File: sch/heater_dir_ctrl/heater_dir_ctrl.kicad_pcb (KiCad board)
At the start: 2 copper layers, 88 parts, among them J1 JMP1, J10 heater, J11 heater, J2 JMP1, J3 UV, J4 SWD, J5 motor, J6 motor, J7 ., J8 ac_in, J9 ac_in, Q1 AO3400, Q2 DTD114E, Q3 Q_Photo_NPN_CE, Q4 2N60, Q5 2N60, Q6 2N60, Q7 2N60, Q8 DTD114E, Q9 DTD114E, SW1 SW_Push, SW2 SW_Push, U1 STM32F031F4P6, U2 LNK306D, U3 AP1117-33, U4 TM1637, U5 IRS2103, U6 LTV-817, U8 IRS2103

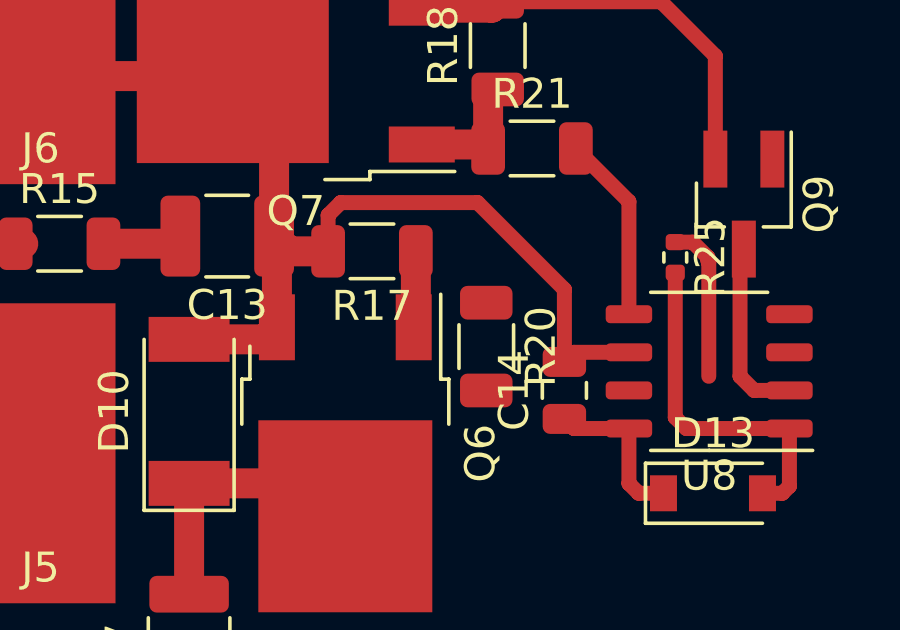
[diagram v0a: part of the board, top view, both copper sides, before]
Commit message: commas
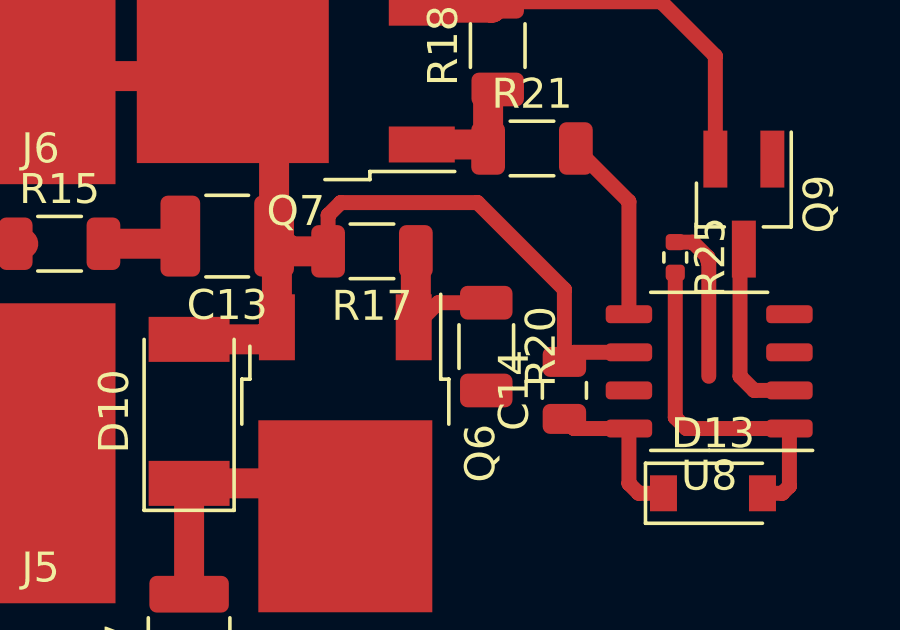
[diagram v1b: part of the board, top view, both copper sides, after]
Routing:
- net Net-(Q6-Pad1): track 2.56 -> 5.32 mm

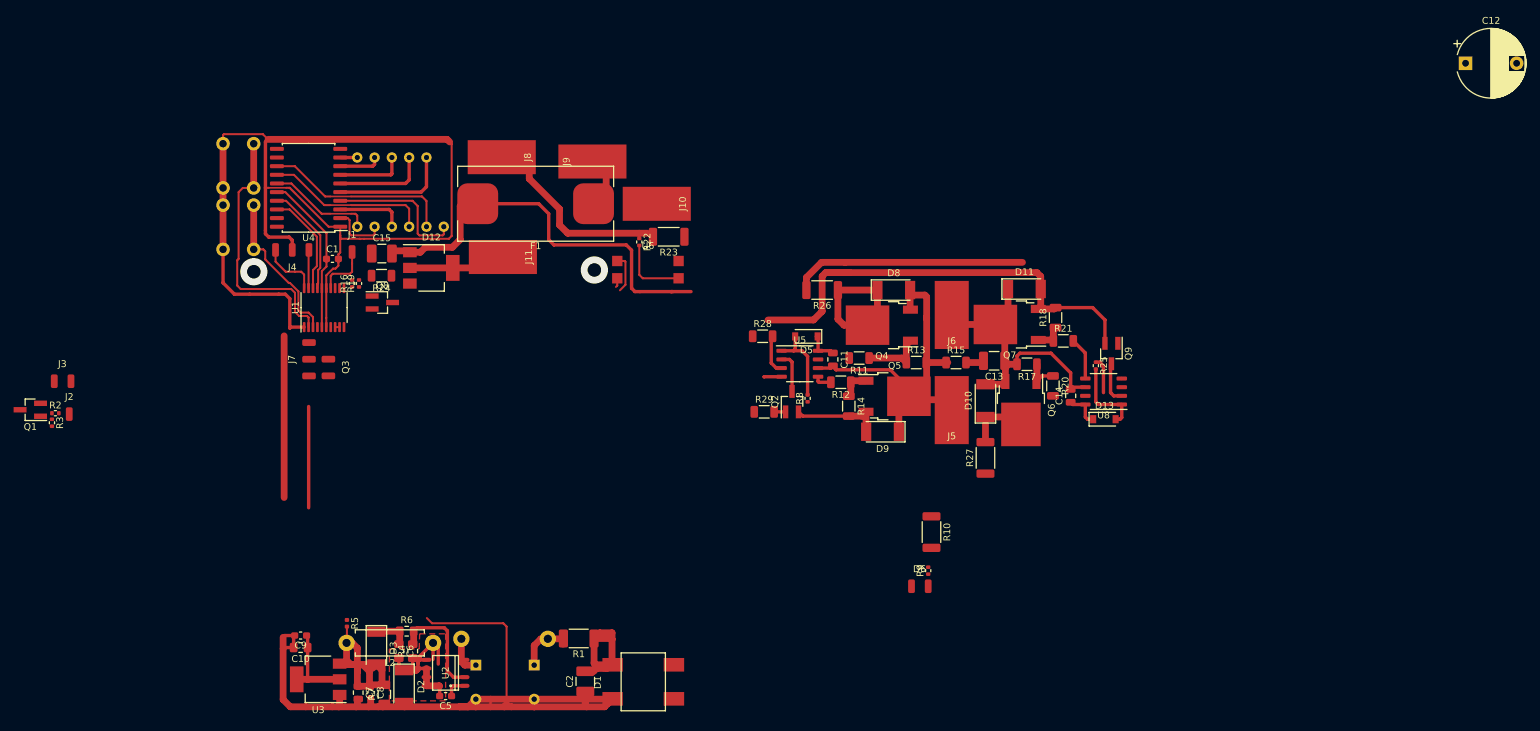
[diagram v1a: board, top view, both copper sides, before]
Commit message: board ok
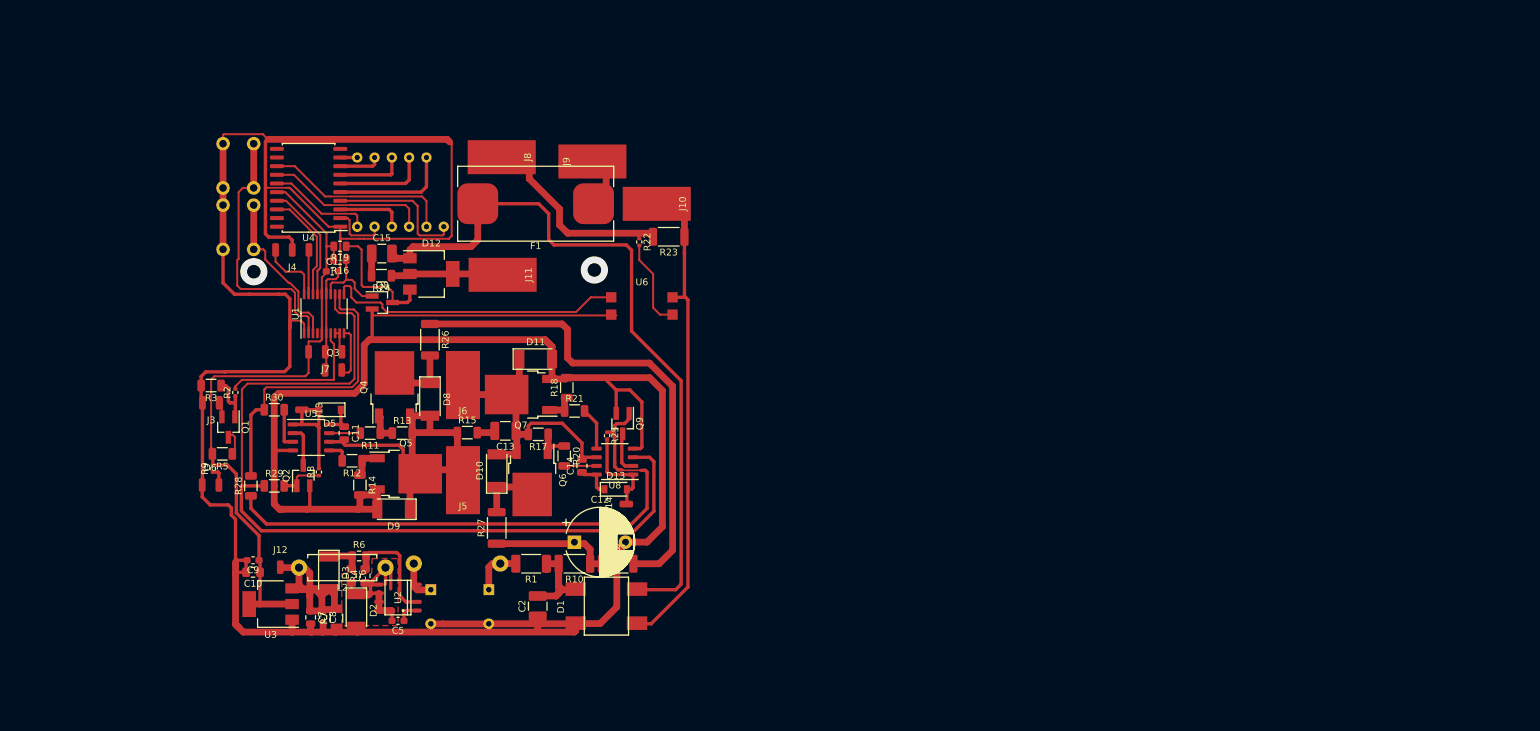
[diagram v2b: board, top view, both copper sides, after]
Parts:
- removed J1, J2: JMP1, Connector_Wire:SolderWirePad_1x01_SMD_1x2mm
- added J12: 10V, Connector_Wire:SolderWirePad_1x01_SMD_1x2mm, F.Cu at (111.9, 125.2)
- added J13: 10V, Connector_Wire:SolderWirePad_1x01_SMD_1x2mm, F.Cu at (115.1, 102.1)
- added J14: 10V, Connector_Wire:SolderWirePad_1x01_SMD_1x2mm, F.Cu at (162.7, 116.0)
- added R30: 220, Resistor_SMD:R_1206_3216Metric, F.Cu at (111.0, 102.1)
- added R31: 1, Resistor_SMD:R_2010_5025Metric, F.Cu at (161.4, 124.7)
- R16, R19: footprint Resistor_SMD:R_0402_1005Metric -> Resistor_SMD:R_0805_2012Metric
- R3, R5: footprint Resistor_SMD:R_0402_1005Metric -> Resistor_SMD:R_1206_3216Metric
- moved C12 148.5 mm to (155.1, 121.5)
- moved R9 106.1 mm to (102.0, 110.7)
- moved D6 105.2 mm to (101.6, 113.2)
- moved R28 78.3 mm to (107.6, 113.3), turned to 90 degrees
- moved R13 76.2 mm to (129.8, 105.5)
- moved R29 72.7 mm to (111.0, 113.3)
- moved R14 72.7 mm to (123.6, 113.2)
- moved D9 72.7 mm to (128.5, 116.7)
- moved R12 72.7 mm to (122.4, 109.6)
- moved Q5 72.7 mm to (130.3, 111.5)
- moved R11 72.6 mm to (125.1, 105.5)
- moved Q2 72.6 mm to (115.3, 111.8)
- moved C11 72.6 mm to (121.3, 105.5)
- moved R8 72.6 mm to (117.6, 111.3)
- moved U5 72.6 mm to (116.4, 106.2)
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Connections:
- R2 pad 2: Net-(J2-Pad1) -> Net-(R2-Pad2)
- R26 pad 1: Net-(D8-Pad1) -> Net-(R26-Pad1)
- R26 pad 2: Net-(C12-Pad1) -> Net-(D8-Pad1)
- R28 pad 2: Net-(R28-Pad2) -> /LEFTO
- R5 pad 2: +10V -> +3V3
- U1 pad 10: Net-(U1-Pad10) -> Net-(Q3-Pad2)
- U1 pad 12: Net-(U1-Pad12) -> /LEFTO
- U1 pad 13: Net-(U1-Pad13) -> /RIGHT
- U1 pad 14: Net-(J1-Pad1) -> Net-(Q8-Pad1)
- U1 pad 7: Net-(U1-Pad7) -> Net-(R2-Pad2)
- U5 pad 3: Net-(R28-Pad2) -> Net-(R30-Pad2)
- U6 pad 4: Net-(U6-Pad4) -> Net-(U1-Pad11)
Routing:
- net GND: track 387.5 -> 538.1 mm
- net /RIGHT: track 0.00 -> 126.7 mm
- net /LEFT: track 5.28 -> 84.3 mm
- net Net-(R26-Pad1): track 0.00 -> 72.5 mm
- net LINE: track 18.3 -> 87.4 mm
- net Net-(U1-Pad11): track 0.00 -> 43.9 mm
- net +3V3: track 51.6 -> 95.5 mm
- net /LEFTO: track 0.00 -> 43.5 mm
- net NEUT: track 66.7 -> 106.6 mm
- net Net-(R2-Pad2): track 0.00 -> 22.3 mm
- net Net-(D12-Pad3): track 0.00 -> 18.4 mm
- net Net-(C12-Pad1): track 34.5 -> 17.9 mm
- net Net-(Q8-Pad1): track 0.00 -> 12.4 mm
- net Net-(D8-Pad1): track 20.6 -> 9.87 mm
- net Net-(Q1-Pad1): track 0.00 -> 10.2 mm
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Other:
- net class Default: clearance 0.5 -> 0.24
- rule trace_clearance: 0.5 -> 0.24
